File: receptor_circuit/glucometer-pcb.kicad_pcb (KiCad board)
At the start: 2 copper layers, 231.6 x 145.8 mm, 168 parts

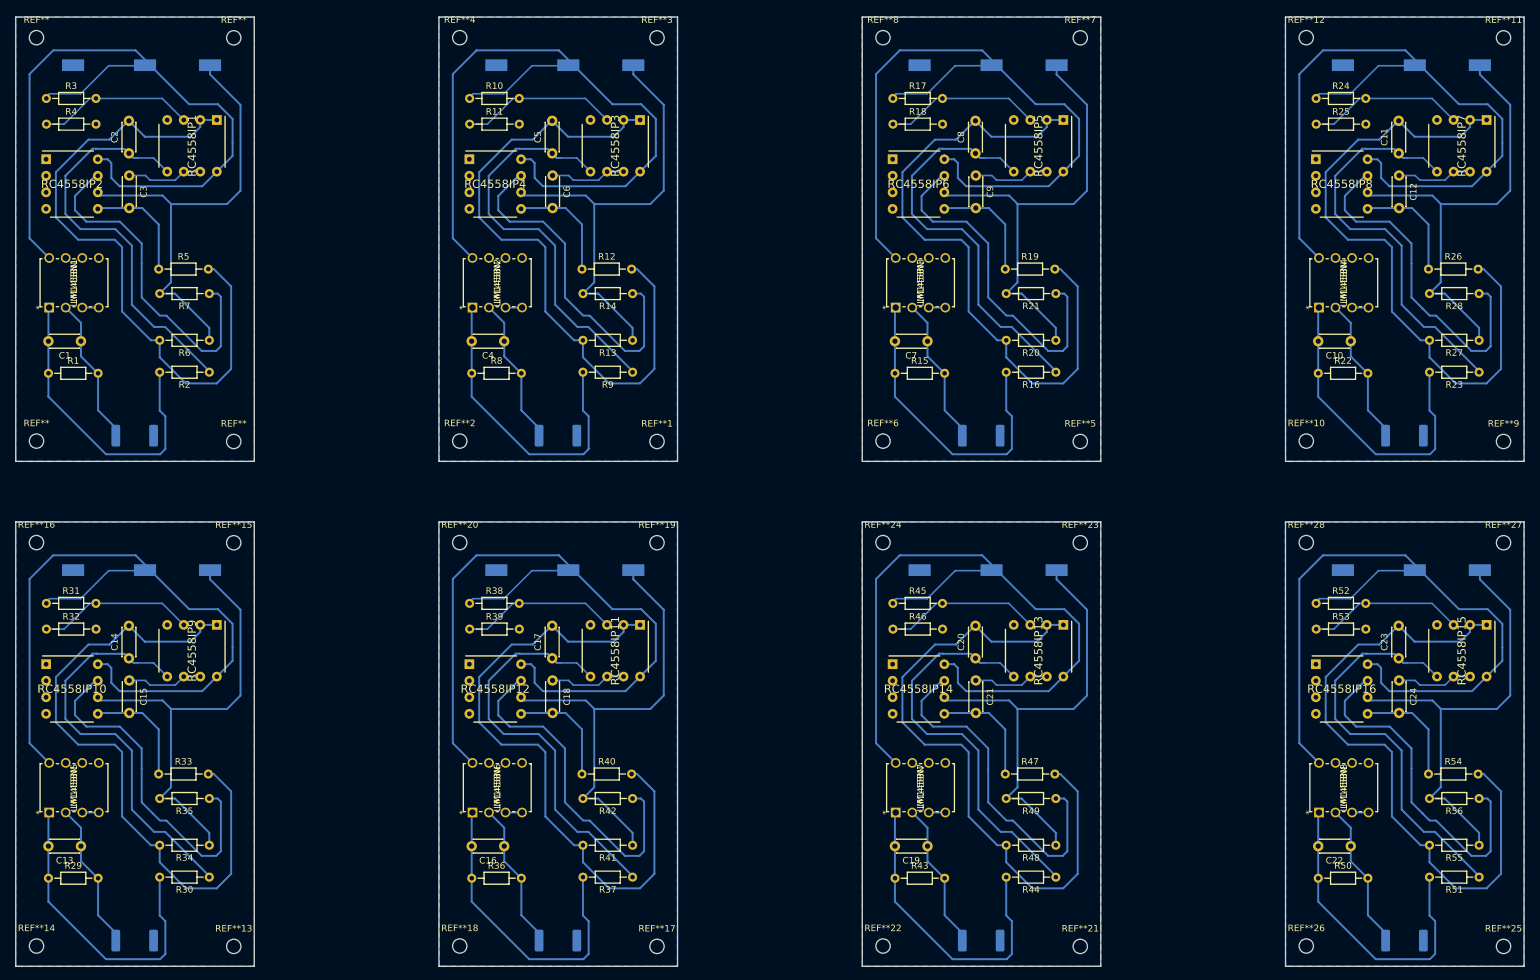
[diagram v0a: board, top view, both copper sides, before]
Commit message: pcb update
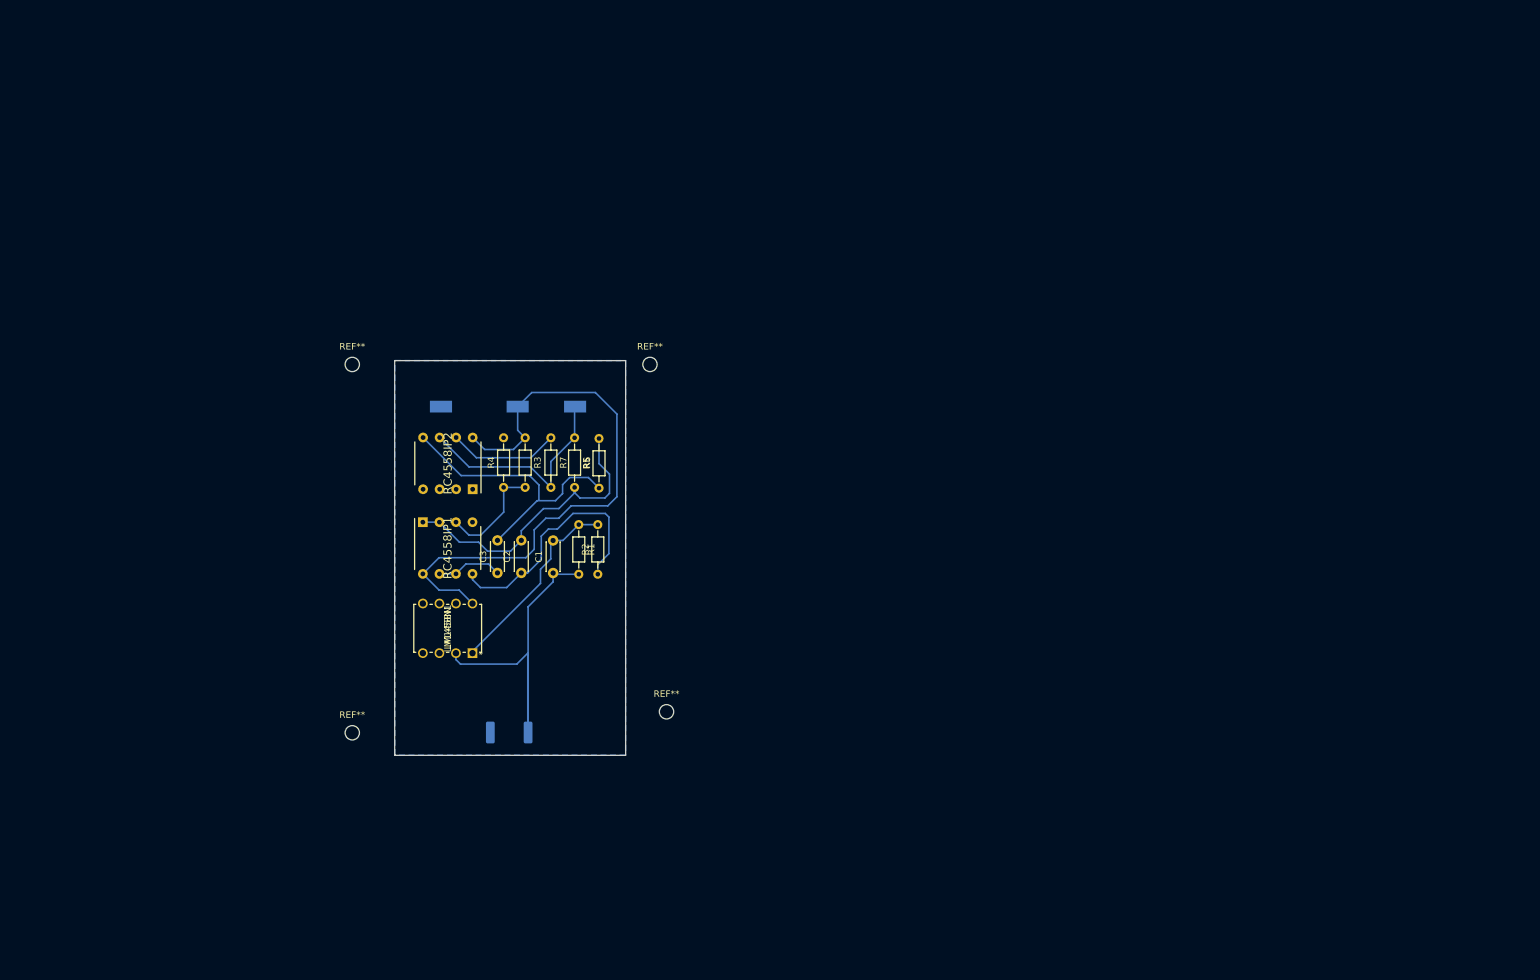
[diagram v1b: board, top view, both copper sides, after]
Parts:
- removed C10, C13, C16, C19, C22, C4, C7: 15p, Capacitor_THT:C_Disc_D4.3mm_W1.9mm_P5.00mm
- removed C11, C14, C17, C20, C23, C5, C8: 100n, Capacitor_THT:C_Disc_D4.3mm_W1.9mm_P5.00mm
- removed C12, C15, C18, C21, C24, C6, C9: 10u, Capacitor_THT:C_Disc_D4.3mm_W1.9mm_P5.00mm
- removed GND2, GND3, GND4, GND5, GND6, GND7, GND8, VCC2, VCC3, VCC4, VCC5, VCC6, VCC7, VCC8: TestPoint, TestPoint:TestPoint_Keystone_5015_Micro-Minature
- removed LM1458N2, LM1458N3, LM1458N4, LM1458N5, LM1458N6, LM1458N7, LM1458N8: LM1458N, Custom:MC1458N
- removed R10, R11, R17, R18, R24, R25, R31, R32, R38, R39, R45, R46, R52, R53: 10k, Resistor_THT:R_Axial_DIN0204_L3.6mm_D1.6mm_P7.62mm_Horizontal
- removed R12, R19, R26, R33, R40, R47, R54: 25k, Resistor_THT:R_Axial_DIN0204_L3.6mm_D1.6mm_P7.62mm_Horizontal
- removed R13, R20, R27, R34, R41, R48, R55: 1k, Resistor_THT:R_Axial_DIN0204_L3.6mm_D1.6mm_P7.62mm_Horizontal
- removed R14, R15, R21, R22, R28, R29, R35, R36, R42, R43, R49, R50, R56, R8: 100k, Resistor_THT:R_Axial_DIN0204_L3.6mm_D1.6mm_P7.62mm_Horizontal
- removed R16, R23, R30, R37, R44, R51, R9: 330k, Resistor_THT:R_Axial_DIN0204_L3.6mm_D1.6mm_P7.62mm_Horizontal
- removed RC4558IP10, RC4558IP11, RC4558IP12, RC4558IP13, RC4558IP14, RC4558IP15, RC4558IP16, RC4558IP3, RC4558IP4, RC4558IP5, RC4558IP6, RC4558IP7, RC4558IP8, RC4558IP9: RC4558IP, Custom:DIP794W53P254L959H508Q8N
- removed RECEPTOR_DIODE2, RECEPTOR_DIODE3, RECEPTOR_DIODE4, RECEPTOR_DIODE5, RECEPTOR_DIODE6, RECEPTOR_DIODE7, RECEPTOR_DIODE8: D_Photo, LED_SMD:LED_2512_6332Metric
- removed REF**1, REF**10, REF**11, REF**12, REF**13, REF**14, REF**15, REF**16, REF**17, REF**18, REF**19, REF**2, REF**20, REF**21, REF**22, REF**23, REF**24, REF**25, REF**26, REF**27, REF**28, REF**3, REF**4, REF**5, REF**6, REF**7, REF**8, REF**9: MountingHole_2.2mm_M2_ISO7380, MountingHole:MountingHole_2.2mm_M2_ISO7380
- removed S_OUT2, S_OUT3, S_OUT4, S_OUT5, S_OUT6, S_OUT7, S_OUT8: SIGNAL_OUT, TestPoint:TestPoint_Keystone_5015_Micro-Minature
- moved R3 90.1 mm to (115.4, 79.8), turned to -90 degrees
- moved R4 89.7 mm to (112.1, 87.5), turned to 90 degrees
- moved C2 88.2 mm to (114.9, 100.6)
- moved R1 84.7 mm to (123.7, 93.2), turned to -90 degrees
- moved C3 83.2 mm to (111.2, 100.6), turned to 90 degrees
- moved REF** 81.2 mm to (134.6, 68.6)
- moved C1 80.8 mm to (119.7, 100.6), turned to 90 degrees
- moved REF** 78.4 mm to (137.2, 121.9)
- moved LM1458N1 77.9 mm to (107.4, 102.8), turned to -90 degrees
- moved VCC1 77.6 mm to (114.3, 75.1)
- moved GND1 77.1 mm to (102.5, 75.1)
- moved S_OUT1 76.8 mm to (123.1, 75.1)
- moved R5 75.5 mm to (126.8, 87.6), turned to 90 degrees
- moved RECEPTOR_DIODE1 73.4 mm to (113.0, 125.1), turned to 0 degrees
- moved RC4558IP1 73.2 mm to (103.6, 96.8), turned to 90 degrees
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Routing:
- net VCC: track 926.2 -> 91.1 mm
- net /PWD_1.65: track 805.1 -> 47.1 mm
- net Net-(R6-Pad1): track 567.3 -> 35.7 mm
- net /SIGNAL_1: track 497.7 -> 38.8 mm
- net Net-(R7-Pad1): track 423.4 -> 17.1 mm
- net Net-(C1-Pad2): track 382.8 -> 30.3 mm
- net Net-(R3-Pad2): track 192.7 -> 16.7 mm
- net Net-(C1-Pad1): track 183.0 -> 55.3 mm
- net /SIGNAL_2: track 138.5 -> 44.2 mm
- net Net-(C3-Pad1): track 93.9 -> 10.1 mm
- net GND: track 25.2 -> 0.09 mm
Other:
- board size 231.6 x 145.8 mm -> 35.5 x 60.6 mm

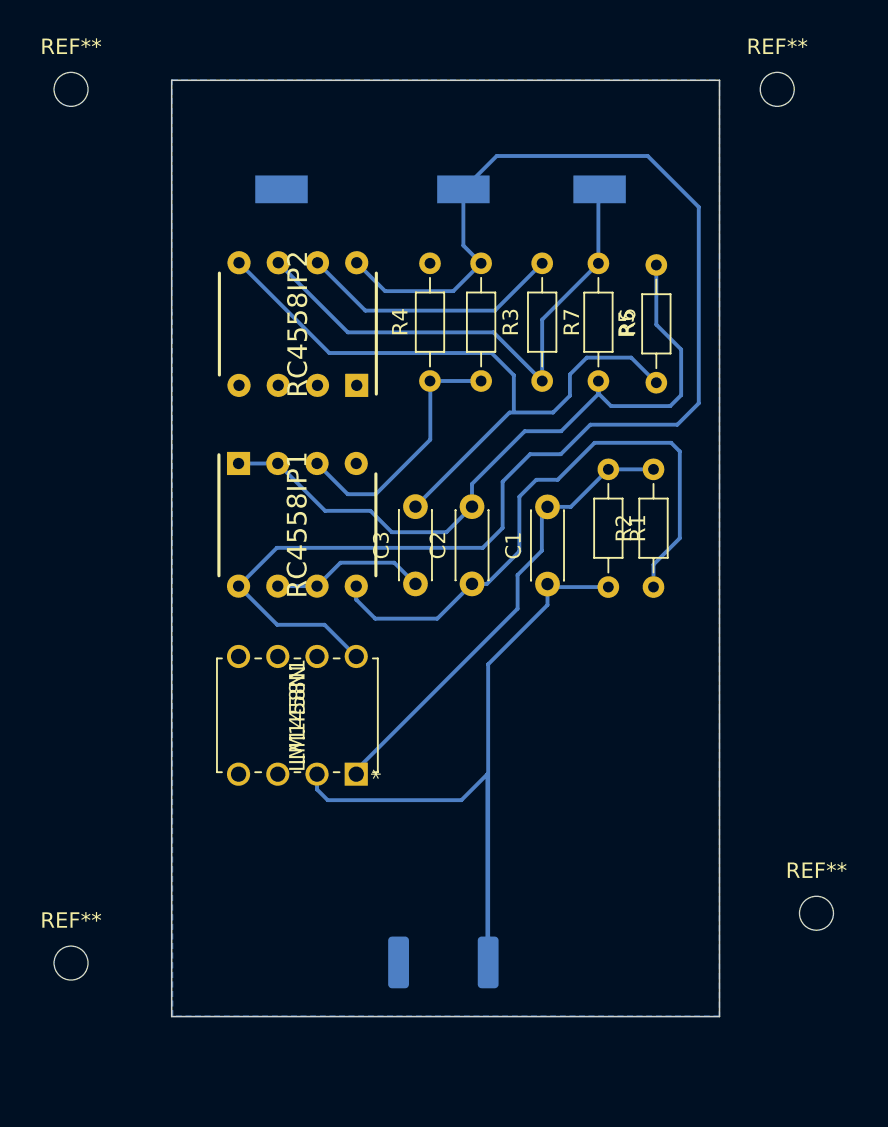
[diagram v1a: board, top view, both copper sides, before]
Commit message: rework receptor PCB
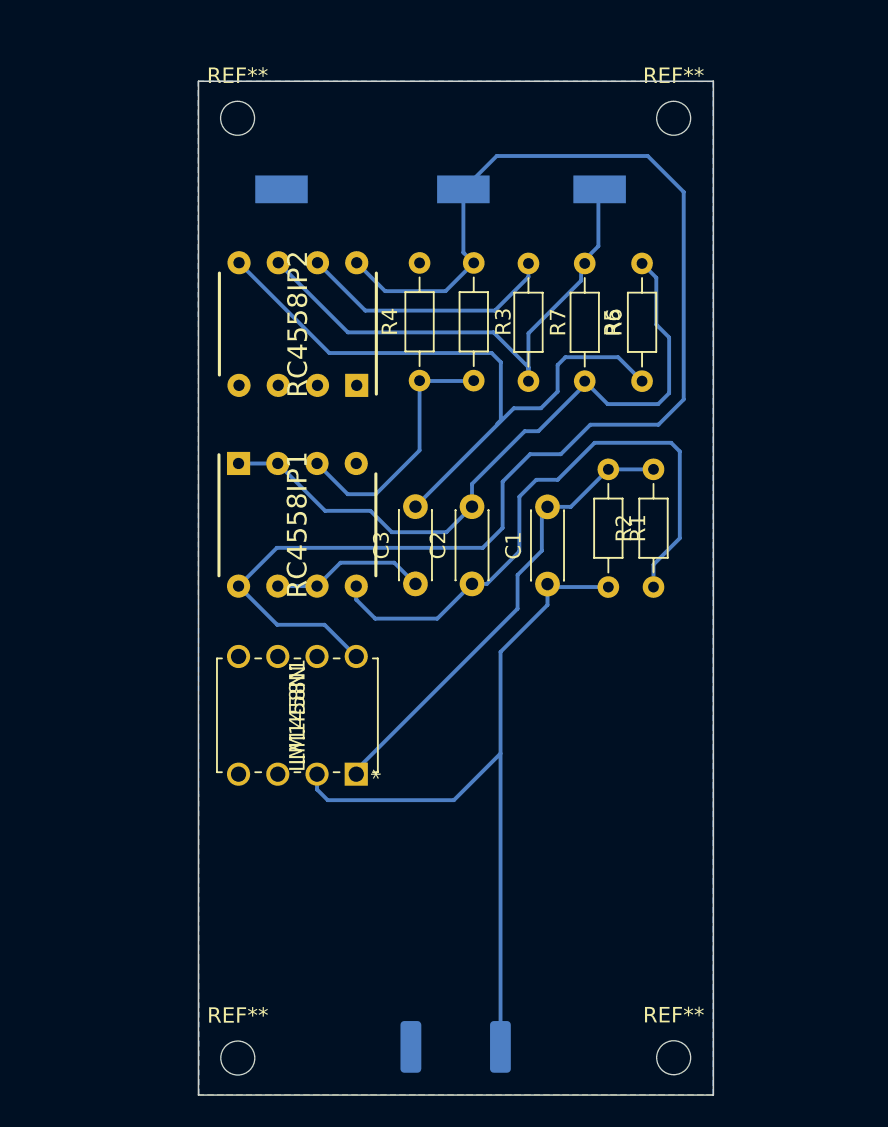
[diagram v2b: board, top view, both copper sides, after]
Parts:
- moved REF** 13.2 mm to (127.9, 131.3)
- moved REF** 12.4 mm to (99.7, 131.3)
- moved REF** 10.9 mm to (99.7, 70.5)
- moved REF** 6.96 mm to (127.9, 70.5)
- moved RECEPTOR_DIODE1 5.53 mm to (113.8, 130.6)
- moved R5 0.93 mm to (125.9, 87.5)
- moved R7 0.89 mm to (118.5, 79.9)
- moved R6 0.89 mm to (122.2, 79.9)
- moved R4 0.68 mm to (111.5, 87.4)
- moved R3 0.48 mm to (115.0, 79.8)
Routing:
- net Net-(C1-Pad1): track 55.3 -> 49.7 mm
- net /PWD_1.65: track 47.1 -> 44.8 mm
- net VCC: track 91.1 -> 88.9 mm
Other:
- board size 35.5 x 60.6 mm -> 33.3 x 65.6 mm
